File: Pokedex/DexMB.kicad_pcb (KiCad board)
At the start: 2 copper layers, 182.6 x 81.3 mm, 21 parts

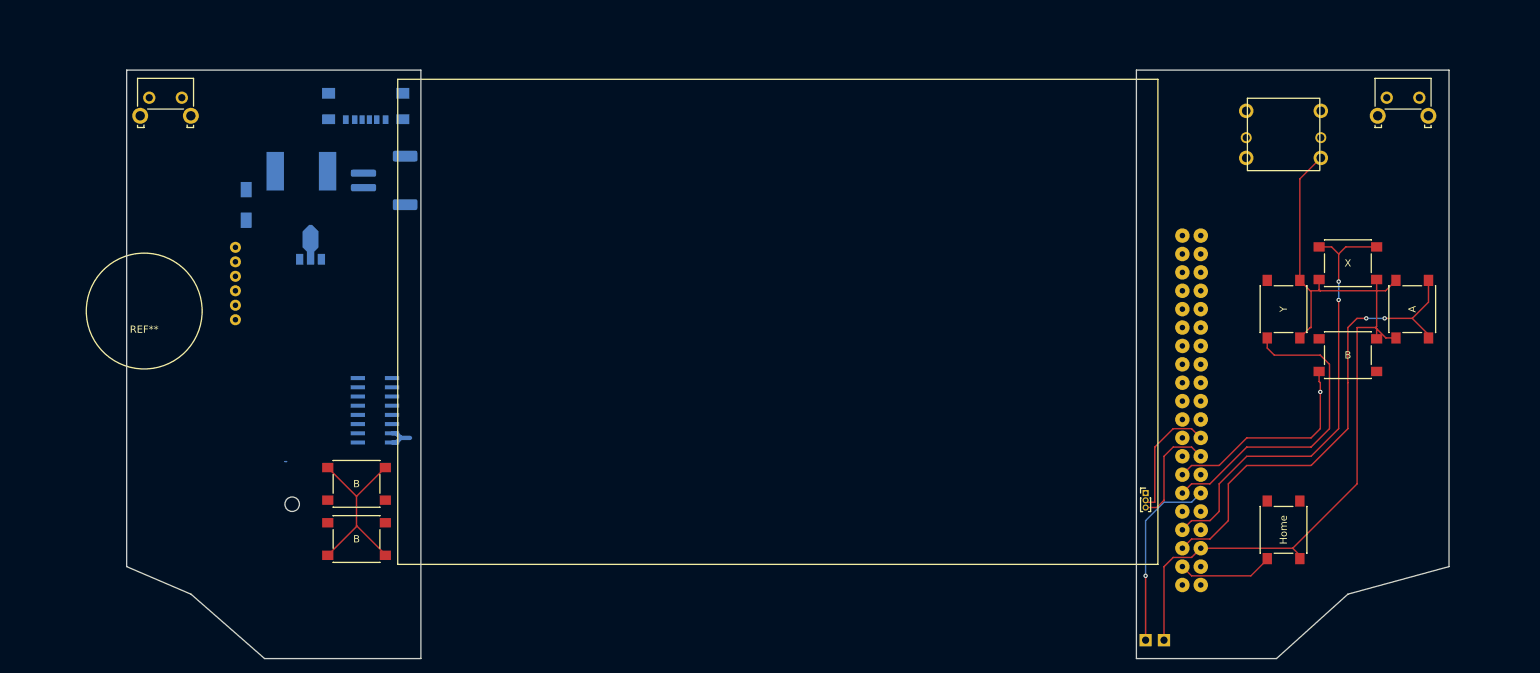
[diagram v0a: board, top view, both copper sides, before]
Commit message: 95% Complete Design
* Looking to add physical flip-flop switch in for power button
* Make pinouts for usb transfer
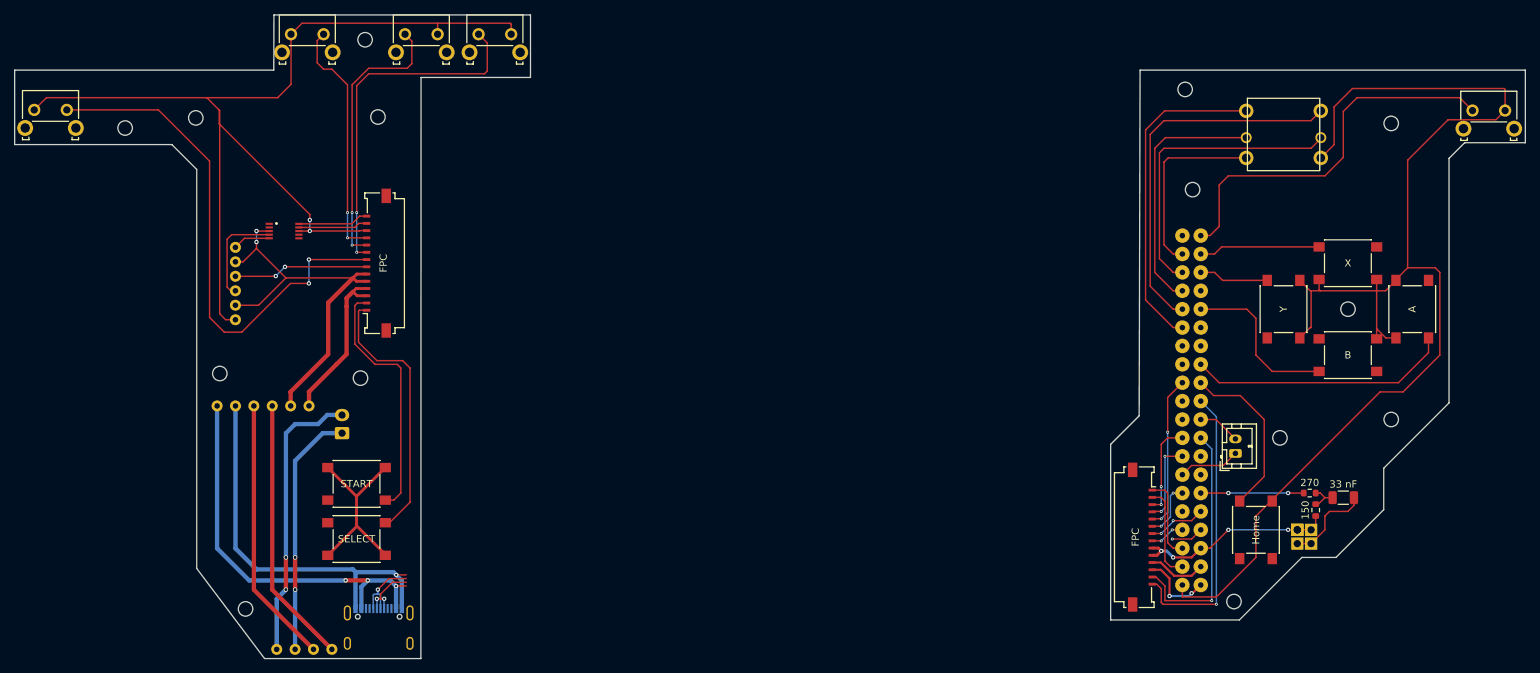
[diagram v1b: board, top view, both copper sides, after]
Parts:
- removed the REF** at (100.6, 63.5)
- removed the REF** at (84.0, 78.3)
- removed the REF** at (91.7, 73.7)
- removed the REF** at (208.3, 118.1)
- removed the REF** at (103.1, 74.9)
- removed the REF** at (92.9, 83.8)
- removed the REF** at (101.8, 106.7)
- added 150: R_0603_1608Metric, Resistor_SMD:R_0603_1608Metric, F.Cu at (231.8, 120.5)
- added 270: R_0603_1608Metric, Resistor_SMD:R_0603_1608Metric, F.Cu at (230.9, 118.1)
- added 33 nF: C_1206_3216Metric, Capacitor_SMD:C_1206_3216Metric, F.Cu at (235.6, 118.7)
- added ? (x2): , , F.Cu at (229.2, 123.2)
- added ?: , , F.Cu at (229.2, 125.1)
- added ADS1115: ADS1115, Custom GBA Tools:MSOP10, F.Cu at (89.3, 81.9)
- added B_Sav: Battery Protection Module, Custom GBA Tools:Battery Protection Module, B.Cu at (97.2, 141.0)
- added Bat_Man: Battery Charger Board, Custom GBA Tools:Battery Charger Board, B.Cu at (78.8, 104.8)
- added Battery: JST_EH_S2B-EH_1x02_P2.50mm_Horizontal, Connector_JST:JST_EH_S2B-EH_1x02_P2.50mm_Horizontal, B.Cu at (97.3, 109.8)
- added FPC: Molex_200528-0140_1x14-1MP_P1.00mm_Horizontal, Connector_FFC-FPC:Molex_200528-0140_1x14-1MP_P1.00mm_Horizontal, F.Cu at (208.3, 124.2)
- added FPC: Molex_200528-0140_1x14-1MP_P1.00mm_Horizontal, Connector_FFC-FPC:Molex_200528-0140_1x14-1MP_P1.00mm_Horizontal, F.Cu at (101.6, 86.4)
- added REF**: SW_Tactile_SKHH_Angled, Button_Switch_THT:SW_Tactile_SKHH_Angled, F.Cu at (90.2, 54.7)
- added REF**: SW_Tactile_SKHH_Angled, Button_Switch_THT:SW_Tactile_SKHH_Angled, F.Cu at (106.0, 54.7)
- added REF**: SW_Tactile_SKHH_Angled, Button_Switch_THT:SW_Tactile_SKHH_Angled, F.Cu at (116.2, 54.7)
- added REF**: JST_PH_B2B-PH-K_1x02_P2.00mm_Vertical, Connector_JST:JST_PH_B2B-PH-K_1x02_P2.00mm_Vertical, F.Cu at (220.7, 112.6)
- added USB C: USB_C_Receptacle_G-Switch_GT-USB-7010ASV, Connector_USB:USB_C_Receptacle_G-Switch_GT-USB-7010ASV, B.Cu at (102.3, 137.8)
- moved ? 26.5 mm to (231.1, 125.1)
- moved ? 25.4 mm to (231.1, 123.2)
- moved REF** 16.0 mm to (54.8, 65.2)
- moved REF** 12.0 mm to (253.4, 65.3)
- moved Home 3.81 mm to (223.5, 123.2)
- renumbered B to SELECT, B to START
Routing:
- net (no net): track 424.7 -> 1644.5 mm, vias 6 -> 48
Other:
- board size 182.6 x 81.3 mm -> 208.7 x 88.9 mm
- board text added: "GND"
- board text added: "VCC"
- board text removed: "3.3V"
